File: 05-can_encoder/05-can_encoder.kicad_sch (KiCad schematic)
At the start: 14 parts, among them IC1 STM32F072CBT6, IC2 AS5047P-ATSM, U1 SN65HVD230DR, U2 LM3940IMPX-3.3_NOPB

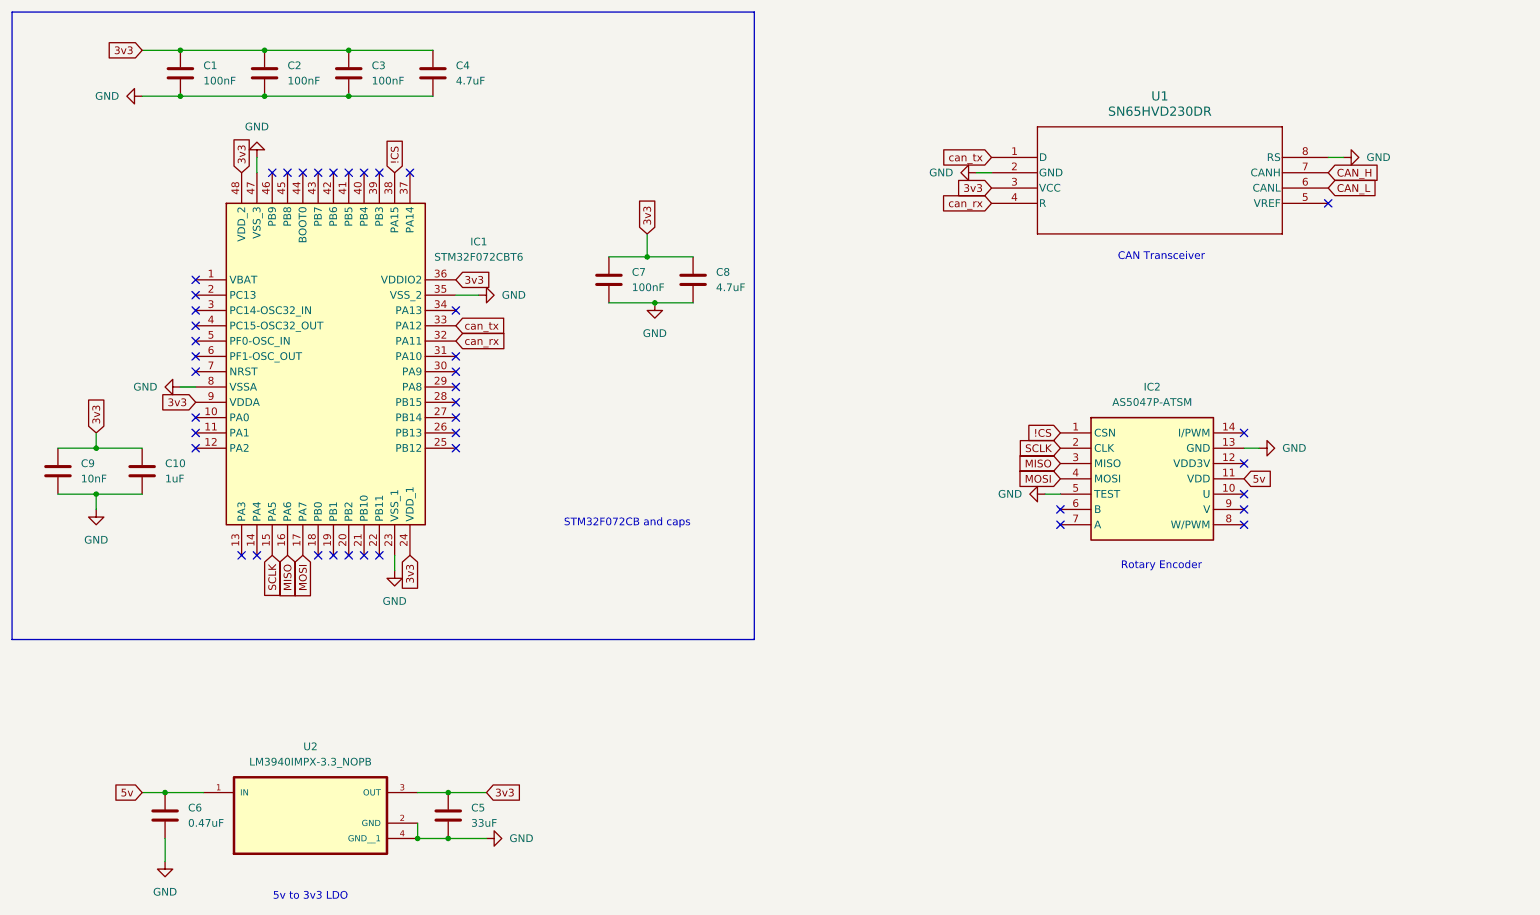
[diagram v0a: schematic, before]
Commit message: layout draft
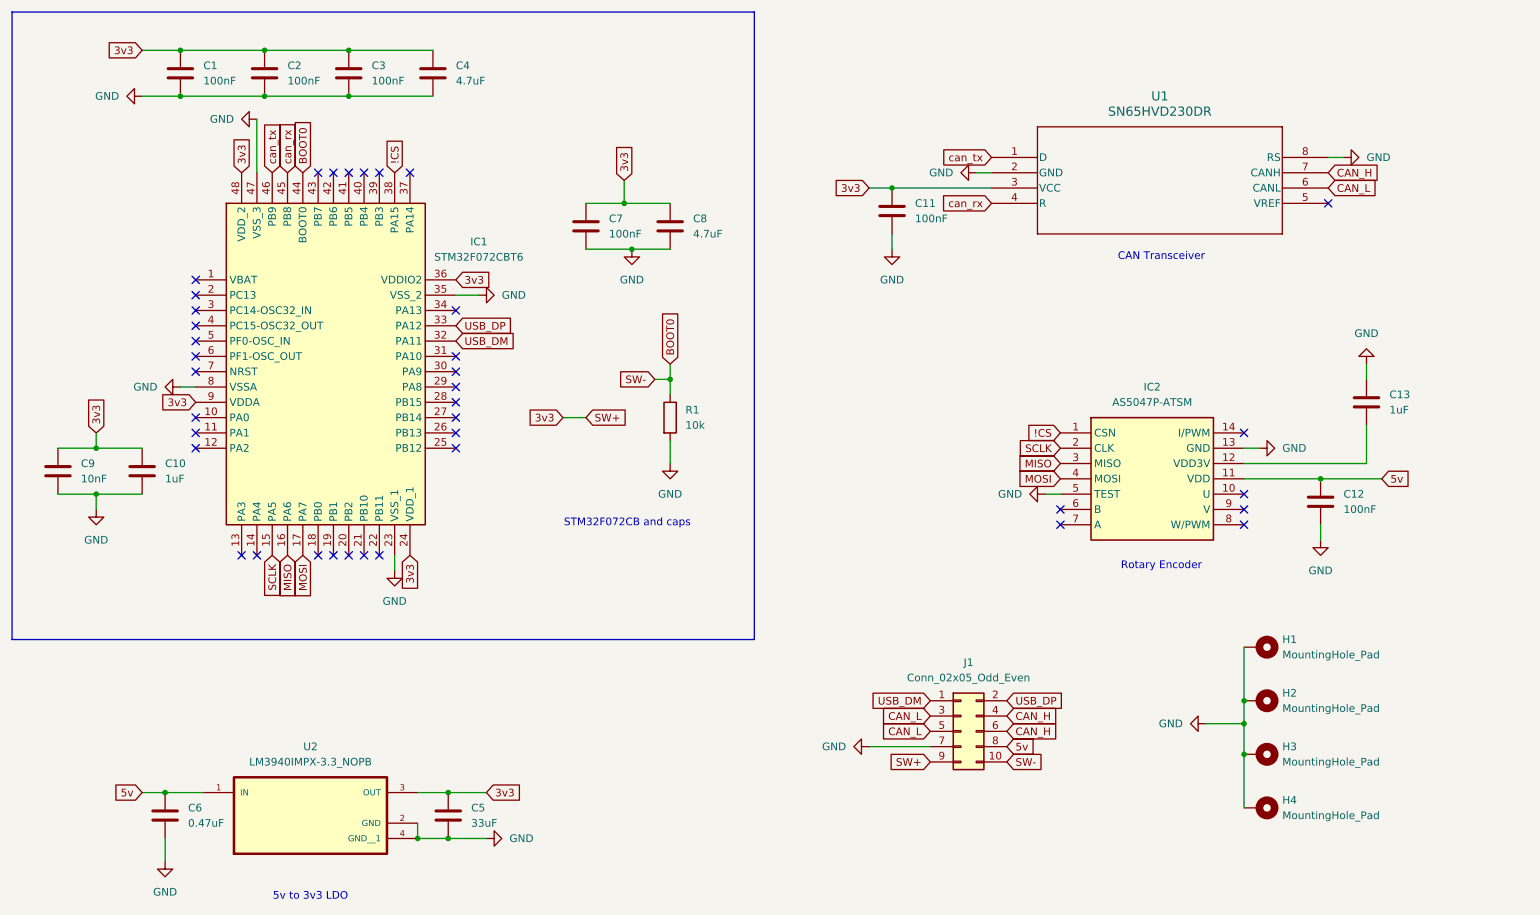
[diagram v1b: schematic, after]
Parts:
- added C11, C12: 100nF, Capacitor_SMD:C_0603_1608Metric, symbol Device:C
- added C13: 1uF, Capacitor_SMD:C_0603_1608Metric, symbol Device:C
- added H1, H2, H3, H4: MountingHole_Pad, MountingHole:MountingHole_2.2mm_M2_DIN965_Pad, symbol Mechanical:MountingHole_Pad
- added J1: Conn_02x05_Odd_Even, Connector_PinHeader_2.54mm:PinHeader_2x05_P2.54mm_Vertical, symbol Connector_Generic:Conn_02x05_Odd_Even
- added R1: 10k, Resistor_SMD:R_0603_1608Metric, symbol Device:R
- C1, C10, C2, C3, C4, C5, C6, C7, C8, C9: footprint (none) -> Capacitor_SMD:C_0603_1608Metric
- IC1: footprint QFP50P900X900X160-48N -> can_encoder:STM32F072CBT6
- IC2: footprint SOP65P640X120-14N -> can_encoder:AS5047P-ATSM
- U1: footprint D8 -> can_encoder:SN65HVD230DR
- U2: footprint LM3940IMPX-3.3_NOPB:SOT230P700X180-4N -> can_encoder:LM3940IMPX
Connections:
- net 3v3: now also C11.1, J1.9 (Pin_9)
- net 5v: now also C12.1, J1.8 (Pin_8)
- net CAN_H: now also J1.4 (Pin_4), J1.6 (Pin_6)
- net CAN_L: now also J1.3 (Pin_3), J1.5 (Pin_5)
- net GND: now also C11.2, C12.2, C13.2, H1.1, H2.1, H3.1, H4.1, J1.7 (Pin_7), R1.2
- net can_rx: now also IC1.45 (PB8); no longer IC1.32 (PA11)
- net can_tx: now also IC1.46 (PB9); no longer IC1.33 (PA12)
- net BOOT0: now reaches IC1.44 (BOOT0)
- net BOOT0: now also J1.10 (Pin_10), R1.1
- net at IC2.12 (VDD3V): now also C13.1
- new net USB_DM: IC1.32 (PA11), J1.1 (Pin_1)
- new net USB_DP: IC1.33 (PA12), J1.2 (Pin_2)
- no-connect marks 42 -> 38
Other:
- moved on the sheet: C7, C8

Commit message: wip layout diff pair
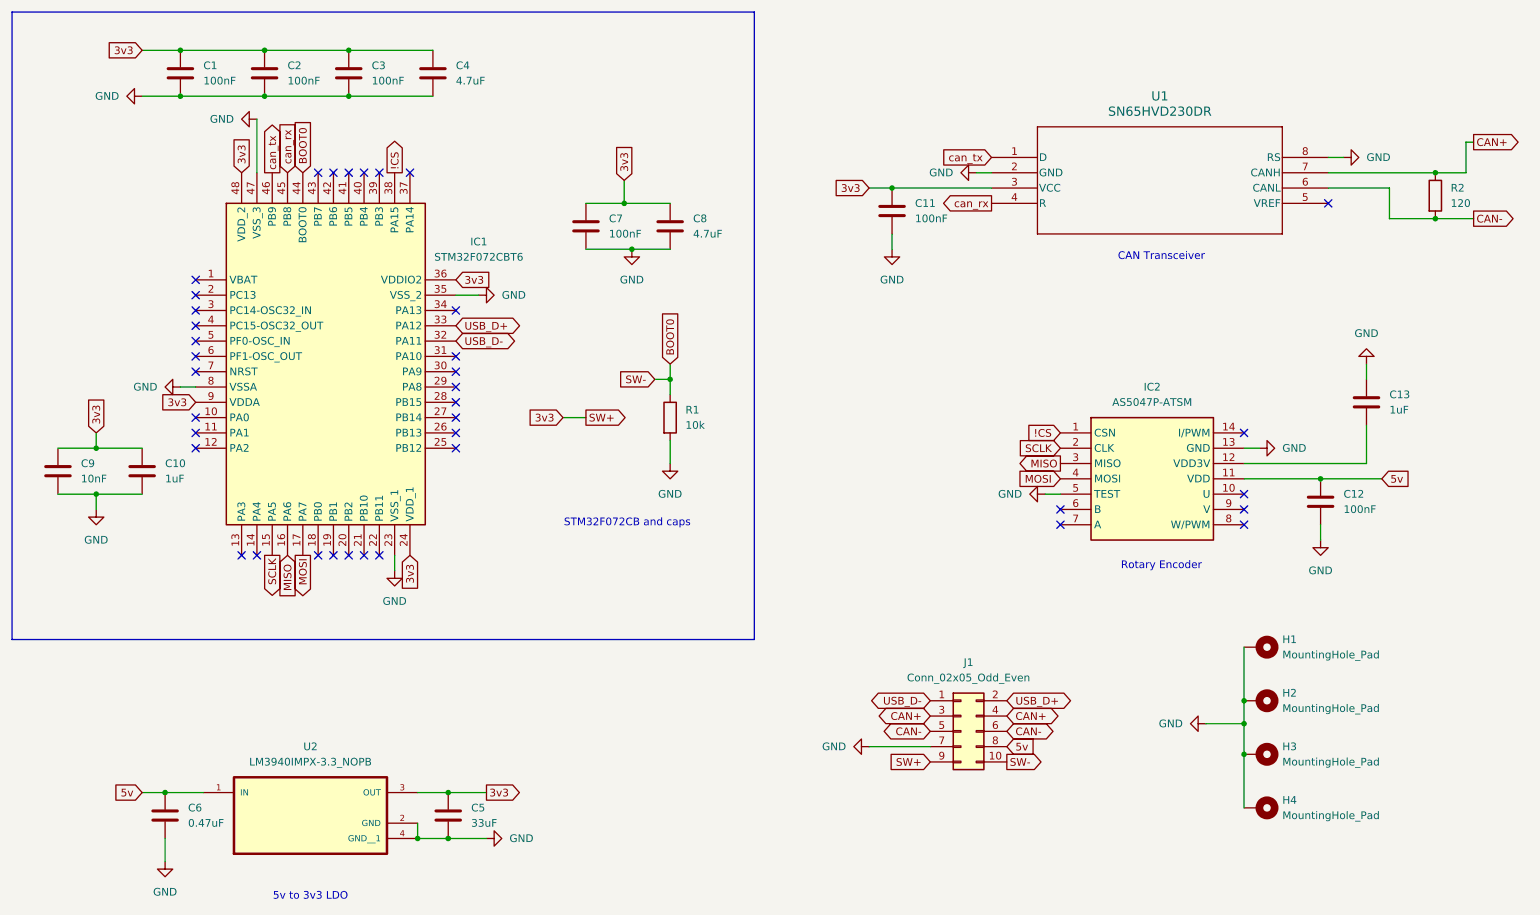
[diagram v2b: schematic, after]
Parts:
- added R2: 120, Resistor_SMD:R_0603_1608Metric, symbol Device:R
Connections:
- net CAN_H renamed CAN+
- net CAN+: now also J1.3 (Pin_3), R2.1; no longer J1.6 (Pin_6)
- net CAN_L renamed CAN-
- net CAN-: now also J1.6 (Pin_6), R2.2; no longer J1.3 (Pin_3)
- net USB_DM renamed USB_D-
- net USB_DP renamed USB_D+
